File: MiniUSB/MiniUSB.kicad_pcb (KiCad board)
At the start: 2 copper layers, 21.8 x 14.5 mm, 7 parts, among them J1 USB_B_Micro, J2 Conn_01x05

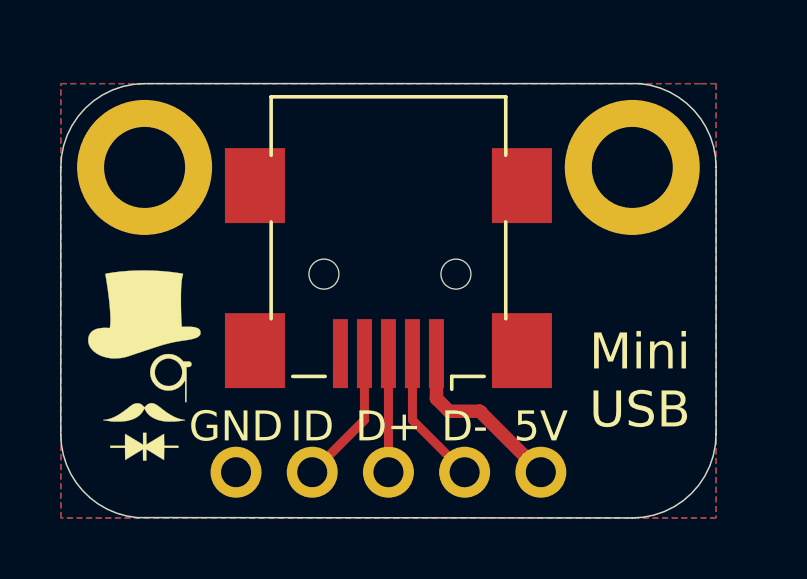
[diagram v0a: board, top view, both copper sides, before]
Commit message: Board Redesign
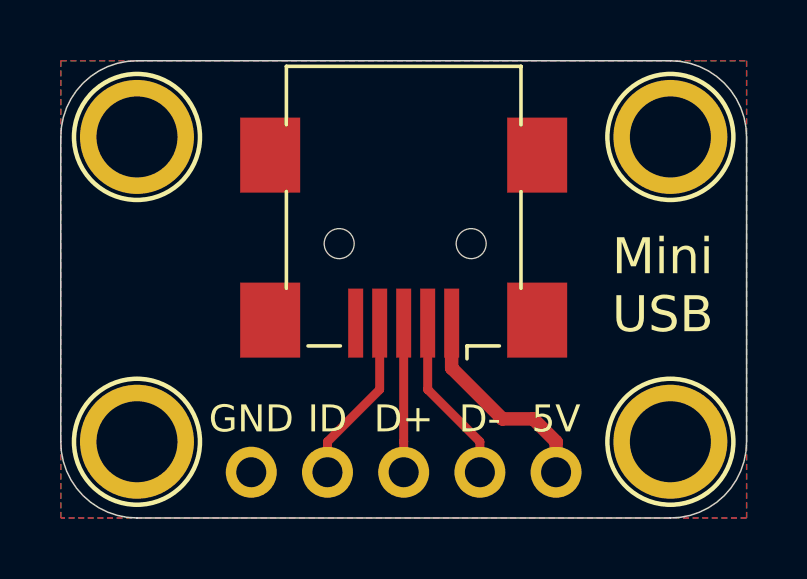
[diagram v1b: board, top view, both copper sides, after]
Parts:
- removed the G*** at (57.4, 34.9)
- removed the H1 at (73.7, 28.3)
- added H1: MountingHole, SirBoardLibrary:MountingHole_M2.5_SirBoard, F.Cu at (74.9, 37.5)
- added H1: MountingHole, SirBoardLibrary:MountingHole_M2.5_SirBoard, F.Cu at (57.1, 37.5)
- added H1: MountingHole, SirBoardLibrary:MountingHole_M2.5_SirBoard, F.Cu at (57.1, 27.3)
- H2: footprint MountingHole:MountingHole_2.7mm_M2.5_ISO14580_Pad -> SirBoardLibrary:MountingHole_M2.5_SirBoard
- J1: value USB_B_Micro -> USB_B_Mini
- moved H2 17.6 mm to (74.9, 27.3), turned to 0 degrees
- moved G*** 1.14 mm to (66.0, 33.7)
- moved J1 1.14 mm to (66.0, 30.9)
- moved G*** 0.81 mm to (66.0, 28.4)
- moved J2 0.51 mm to (71.1, 38.5)
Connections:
- net Net-(J1-Pad1) renamed /VBus
- net Net-(J1-Pad2) renamed /D-
- net Net-(J1-Pad3) renamed /D+
- net Net-(J1-Pad4) renamed /ID
- net Net-(J1-Pad5) renamed /GND
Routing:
- net /VBus: track 5.95 -> 6.96 mm
- net /D+: track 3.90 -> 4.92 mm
- net /ID: track 4.62 -> 5.64 mm
- net /D-: track 4.62 -> 5.64 mm
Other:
- board size 21.8 x 14.5 mm -> 22.9 x 15.2 mm
- board text added: "www.SirBoard.com"
